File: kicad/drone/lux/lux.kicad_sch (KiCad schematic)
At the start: 33 parts, among them J1 mpu6500, J2 usb, J3 battery, M1 cw1, M2 cww1, M3 cw2, M4 cww1, U1 ESP32-S3-WROOM-1U-N16R8, U2 BL5612, U3 BL5612, U4 BL5612, U5 TPS63020DSJR

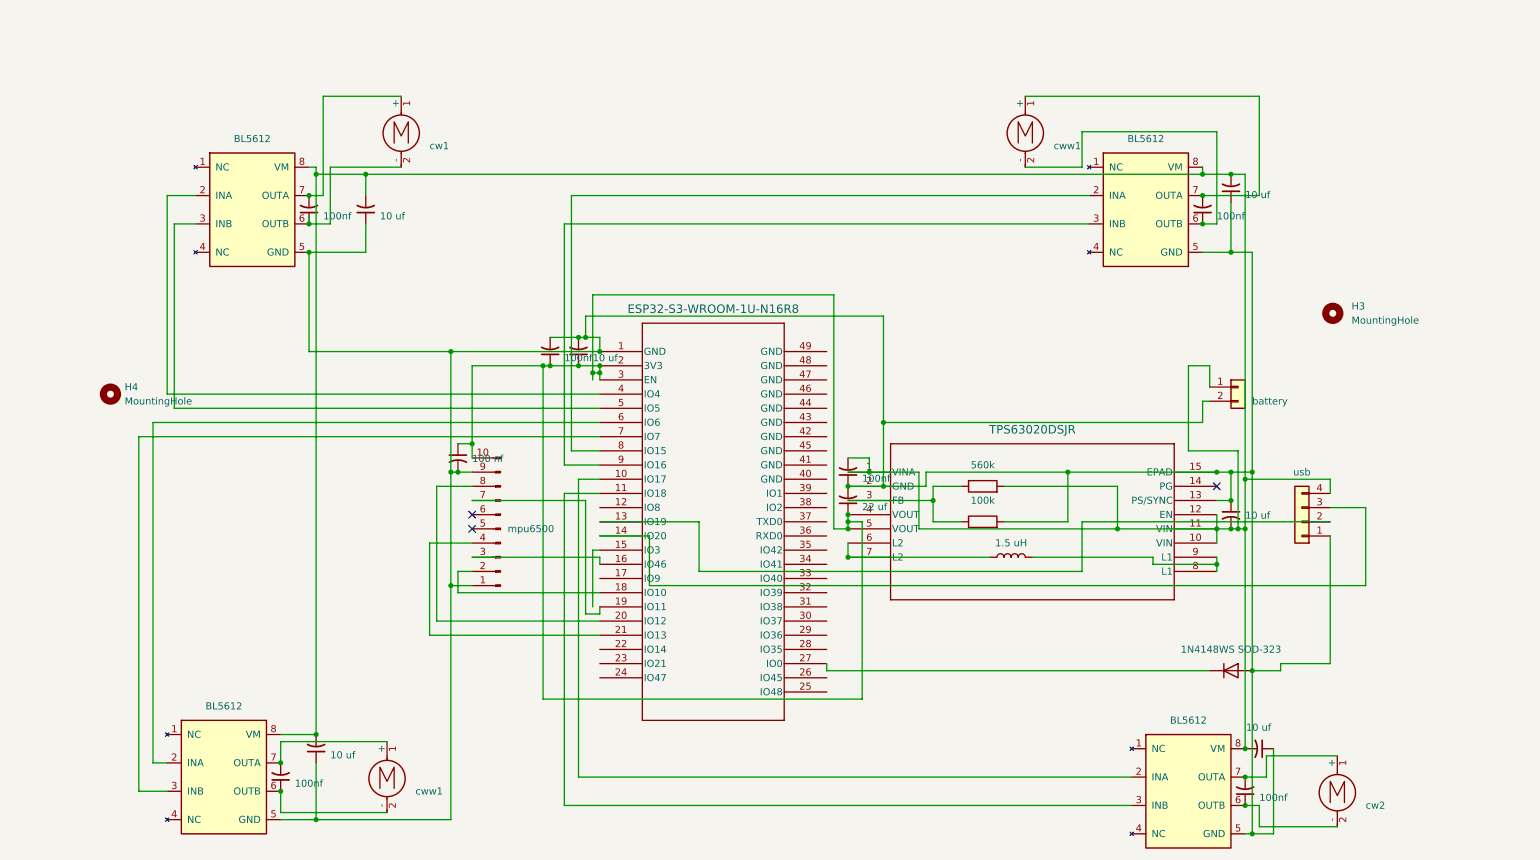
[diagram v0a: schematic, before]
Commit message: sept 12
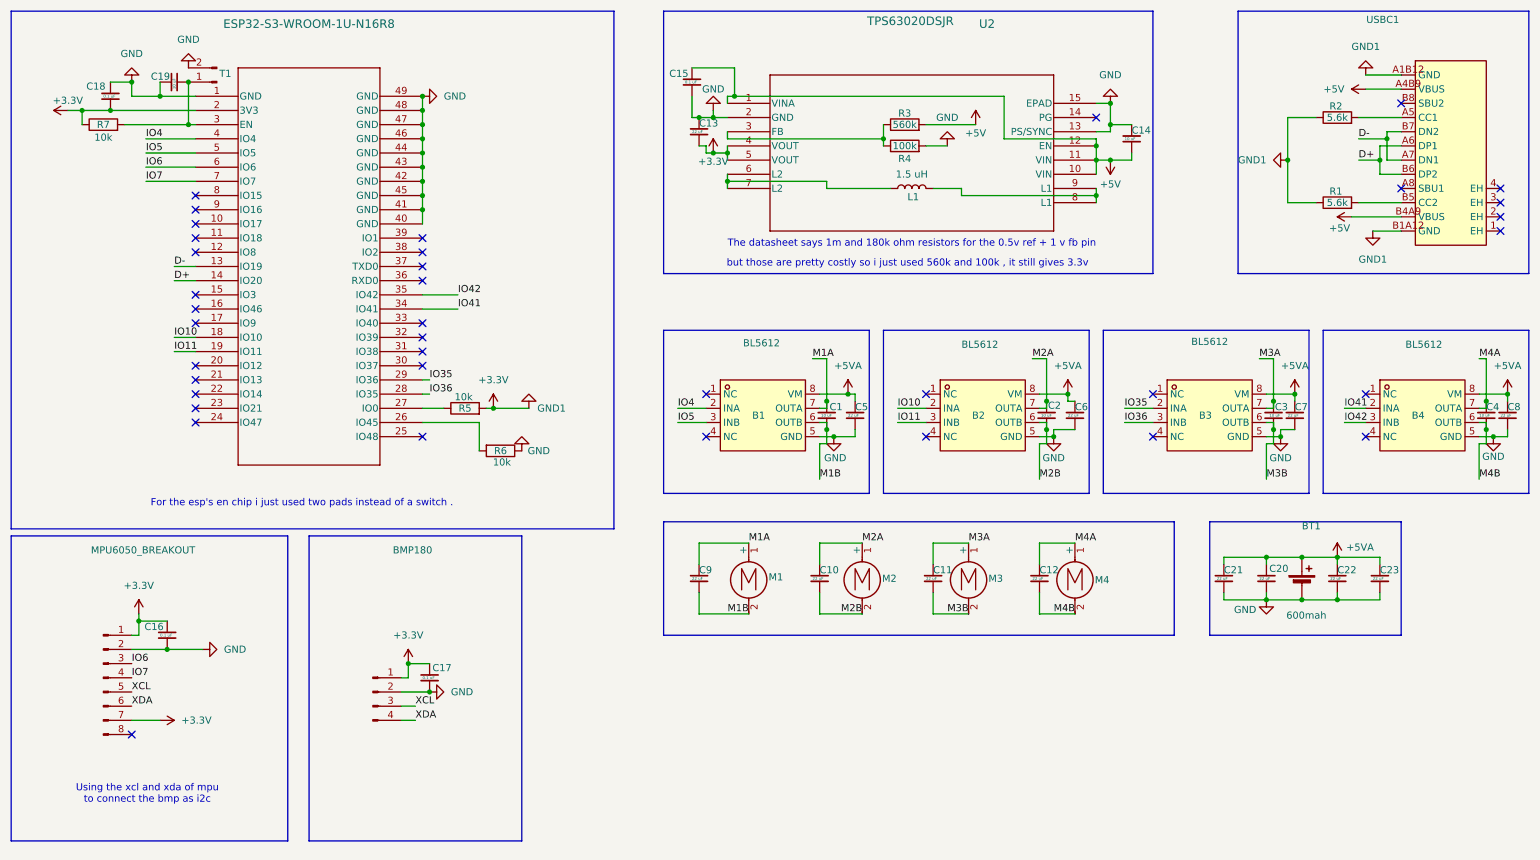
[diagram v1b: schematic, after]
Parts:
- removed C1, C14, C2, C3, C4, C5: 100nf, Capacitor_SMD:C_0402_1005Metric, symbol Device:C_Small_US
- removed C10: 100 nf, Capacitor_SMD:C_0402_1005Metric, symbol Device:C_Small_US
- removed C11, C13, C6, C7, C8, C9: 10 uf, Capacitor_SMD:C_0805_2012Metric, symbol Device:C_Small_US
- removed C12: 22 uf, Capacitor_SMD:C_1206_3216Metric, symbol Device:C_Small_US
- removed D1: 1N4148WS SOD-323, Diode_SMD:D_SOD-323, symbol Device:D
- removed H3, H4: MountingHole, MountingHole:MountingHole_2.5mm, symbol Mechanical:MountingHole
- removed J1: mpu6500, Connector_Hirose:Hirose_DF13-10P-1.25DSA_1x10_P1.25mm_Vertical, symbol Connector:Conn_01x10_Pin
- removed J2: usb, Connector_Hirose:Hirose_DF13-04P-1.25DSA_1x04_P1.25mm_Vertical, symbol Connector_Generic:Conn_01x04
- removed J3: battery, Connector:JWT_A3963_1x02_P3.96mm_Vertical, symbol Connector_Generic:Conn_01x02
- removed U2, U3, U4, b1: BL5612, Package_SO:SOIC-8_3.9x4.9mm_P1.27mm, symbol BL5612:BL5612
- removed U5: TPS63020DSJR, footprints:DSJ14_2P85X1P58, symbol 2026-09-04_08-16-50:TPS63020DSJR
- added B1, B2, B3, B4: BL5612, easyeda2kicad:SOP-8_L4.9-W3.9-P1.27-LS6.0-BL, symbol bl56:BL5612
- added BMP: BMP180, Connector:FanPinHeader_1x04_P2.54mm_Vertical, symbol Connector:Conn_01x04_Pin
- added BT1: 600mah, Connector_PinHeader_2.54mm:PinHeader_1x02_P2.54mm_Vertical, symbol Device:Battery_Cell
- added C1, C14, C19, C2, C3, C4: 10 uF, Capacitor_SMD:C_0805_2012Metric, symbol Device:C_Small
- added C10, C11, C12, C13, C20, C21, C22, C23, C5, C6, C7, C8, C9: 22 uF, Capacitor_SMD:C_1206_3216Metric, symbol Device:C_Small
- added C15, C16, C17, C18: 0.1 uF, Capacitor_SMD:C_0402_1005Metric, symbol Device:C_Small
- added MPU1: MPU6050_BREAKOUT, Connector_Hirose:Hirose_DF13-08P-1.25DSA_1x08_P1.25mm_Vertical, symbol Connector:Conn_01x08_Pin
- added R3: 560k, Resistor_SMD:R_0603_1608Metric, symbol Device:R
- added R4: 100k, Resistor_SMD:R_0603_1608Metric, symbol Device:R
- added R5, R6, R7: 10k, Module:Pololu_Breakout-16_15.2x20.3mm, symbol Device:R
- added T1: trace, Capacitor_SMD:C_1206_3216Metric, symbol Connector:Conn_01x02_Pin
- added U2: TPS63020DSJR, footprints:DSJ14_2P85X1P58, symbol 2026-09-04_08-16-50:TPS63020DSJR
- added USBC1: TYPE-C-31-M-12, easyeda2kicad:USB-C_SMD-TYPE-C-31-M-12_1, symbol easyeda2kicad:TYPE-C-31-M-12
- L1: footprint Inductor_SMD:L_Bourns-SRN8040_8x8.15mm -> footprints:DSJ14_2P85X1P58
- M1: value cw1 -> Motor_DC; footprint Connector_PinHeader_1.27mm:PinHeader_1x02_P1.27mm_Vertical -> Connector_JST:JST_PH_B2B-PH-K_1x02_P2.00mm_Vertical
- M2, M4: value cww1 -> Motor_DC; footprint Connector_PinHeader_1.27mm:PinHeader_1x02_P1.27mm_Vertical -> Connector_JST:JST_PH_B2B-PH-K_1x02_P2.00mm_Vertical
- M3: value cw2 -> Motor_DC; footprint Connector_PinHeader_1.27mm:PinHeader_1x02_P1.27mm_Vertical -> Connector_JST:JST_PH_B2B-PH-K_1x02_P2.00mm_Vertical
- R1: value 100k -> 5.6k
- R2: value 560k -> 5.6k
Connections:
- net M4A: now reaches M4.1 (+)
- net M4A: now also B4.7 (OUTA), C12.1, C4.1
- net M4B: now reaches M4.2 (-)
- net M4B: now also B4.6 (OUTB), C12.2, C4.2
- net at R1.2: now also USBC1.B5 (CC2); no longer U1.1 (GND)
- net M3B: now reaches M3.2 (-)
- net M3B: now also B3.6 (OUTB), C11.2, C3.2
- net M3A: now reaches M3.1 (+)
- net M3A: now also B3.7 (OUTA), C11.1, C3.1
- net at R2.2: now also USBC1.A5 (CC1)
- net at U1.3 (EN): now also C19.2, R7.2, T1.1 (Pin_1); no longer U1.2 (3V3)
- net IO6: now reaches U1.6 (IO6)
- net IO6: now also MPU1.3 (Pin_3)
- net IO7: now reaches U1.7 (IO7)
- net IO7: now also MPU1.4 (Pin_4)
- net M2B: now reaches M2.2 (-)
- net M2B: now also B2.6 (OUTB), C10.2, C2.2
- net M2A: now reaches M2.1 (+)
- net M2A: now also B2.7 (OUTA), C10.1, C2.1
- net at L1.1: now also U2.6 (L2), U2.7 (L2)
- net at L1.2: now also U2.8 (L1), U2.9 (L1)
- net +3.3V: now reaches R1.1, R2.1
- net +3.3V: now also U1.2 (3V3), BMP.1 (Pin_1), C13.2, C16.1, C17.1, C18.2, MPU1.1 (Pin_1), MPU1.7 (Pin_7), R5.2, R7.1, U2.4 (VOUT), U2.5 (VOUT), USBC1.A1B12 (GND), USBC1.B1A12 (GND)
- net D-: now reaches U1.13 (IO19)
- net D-: now also USBC1.A7 (DN1), USBC1.B7 (DN2)
- net D+: now reaches U1.14 (IO20)
- net D+: now also USBC1.A6 (DP1), USBC1.B6 (DP2)
- net IO10: now reaches U1.18 (IO10)
- net IO10: now also B2.2 (INA)
- net IO11: now reaches U1.19 (IO11)
- net IO11: now also B2.3 (INB)
- net at U1.26 (IO45): now also R6.2
- net at U1.27 (IO0): now also R5.1
- net IO36: now reaches U1.28 (IO35)
- net IO36: now also B3.3 (INB)
- net IO35: now reaches U1.29 (IO36)
- net IO35: now also B3.2 (INA)
- net IO41: now reaches U1.34 (IO41)
- net IO41: now also B4.2 (INA)
- net IO42: now reaches U1.35 (IO42)
- net IO42: now also B4.3 (INB)
- net IO4: now reaches U1.4 (IO4)
- net IO4: now also B1.2 (INA)
- net GND: now reaches U1.40 (GND)
- net GND: now also U1.1 (GND), U1.41 (GND), U1.42 (GND), U1.43 (GND), U1.44 (GND), U1.45 (GND), U1.46 (GND), U1.47 (GND), U1.48 (GND), U1.49 (GND), B1.5 (GND), B2.5 (GND), B3.5 (GND), B4.5 (GND), BMP.2 (Pin_2), BT1.2 (-), C13.1, C14.1, C15.2, C16.2, C17.2, C18.1, C19.1, C20.2, C21.2, C22.2, C23.2, C5.2, C6.2, C7.2, C8.2, MPU1.2 (Pin_2), R4.2, R6.1, T1.2 (Pin_2), U2.13 (PS/SYNC), U2.15 (EPAD), U2.2 (GND)
- net IO5: now reaches U1.5 (IO5)
- net IO5: now also B1.3 (INB)
- net M1B: now reaches M1.2 (-)
- net M1B: now also B1.6 (OUTB), C1.2, C9.2
- net M1A: now reaches M1.1 (+)
- net M1A: now also B1.7 (OUTA), C1.1, C9.1
- new net: R3.1, R4.1, U2.3 (FB)
- new net +5V: C14.2, C15.1, R3.2, U2.1 (VINA), U2.10 (VIN), U2.11 (VIN), U2.12 (EN), USBC1.A4B9 (VBUS), USBC1.B4A9 (VBUS)
- new net +5VA: B1.8 (VM), B2.8 (VM), B3.8 (VM), B4.8 (VM), BT1.1 (+), C20.1, C21.1, C22.1, C23.1, C5.1, C6.1, C7.1, C8.1
- new net XCL: BMP.3 (Pin_3), MPU1.5 (Pin_5)
- new net XDA: BMP.4 (Pin_4), MPU1.6 (Pin_6)
- no-connect marks 3 -> 38
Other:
- note added: "For the esp's en chip i just used two pads instead of a switch ."
- note added: "The datasheet says 1m and 180k ohm resistors for the 0.5v ref + 1 v fb pin"
- note added: "Using the xcl and xda of mpu to connect the bmp as i2c"
- note added: "but those are pretty costly so i just used 560k and 100k , it still gives 3.3v"
- title: (none) -> Luxion

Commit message: sept 13
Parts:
- BMP1: renamed from BMP; footprint Connector:FanPinHeader_1x04_P2.54mm_Vertical -> Connector_Hirose:Hirose_DF13-04P-1.25DSA_1x04_P1.25mm_Vertical
- L1: footprint footprints:DSJ14_2P85X1P58 -> Inductor_SMD:L_Bourns-SRN8040_8x8.15mm
- R5, R6, R7: footprint Module:Pololu_Breakout-16_15.2x20.3mm -> Resistor_SMD:R_0603_1608Metric
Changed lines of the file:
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@@
 			)
 		)
-		(property "Footprint" "footprints:DSJ14_2P85X1P58"
+		(property "Footprint" "Inductor_SMD:L_Bourns-SRN8040_8x8.15mm"
 			(at 173.99 44.45 0)
 			(hide yes)
@@
 			)
 		)
-		(property "Footprint" "Module:Pololu_Breakout-16_15.2x20.3mm"
+		(property "Footprint" "Resistor_SMD:R_0603_1608Metric"
 			(at 29.21 34.798 90)
 			(hide yes)
@@
 			)
 		)
-		(property "Footprint" "Module:Pololu_Breakout-16_15.2x20.3mm"
+		(property "Footprint" "Resistor_SMD:R_0603_1608Metric"
 			(at 93.98 85.598 90)
 			(hide yes)
@@
 			)
 		)
-		(property "Footprint" "Module:Pololu_Breakout-16_15.2x20.3mm"
+		(property "Footprint" "Resistor_SMD:R_0603_1608Metric"
 			(at 100.33 89.662 90)
 			(hide yes)
@@
 		(in_pos_files yes)
 		(dnp no)
-		(property "Reference" "BMP"
+		(property "Reference" "BMP1"
 			(at 79.756 115.062 0)
 			(hide yes)
@@
 			)
 		)
-		(property "Footprint" "Connector:FanPinHeader_1x04_P2.54mm_Vertical"
+		(property "Footprint" "Connector_Hirose:Hirose_DF13-04P-1.25DSA_1x04_P1.25mm_Vertical"
 			(at 77.47 134.62 0)
 			(hide yes)
@@
 			(project "lux"
 				(path "/f3a45523-230c-48ab-a937-ad3e7df8831b"
-					(reference "BMP")
+					(reference "BMP1")
 					(unit 1)
 				)
